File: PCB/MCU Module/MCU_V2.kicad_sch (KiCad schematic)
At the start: 11 parts, among them J2 Conn_01x09_Pin, J3 Conn_01x02_Socket, U1 XIAO-nRF54l15-SMD, U5 MAX17048G_T10

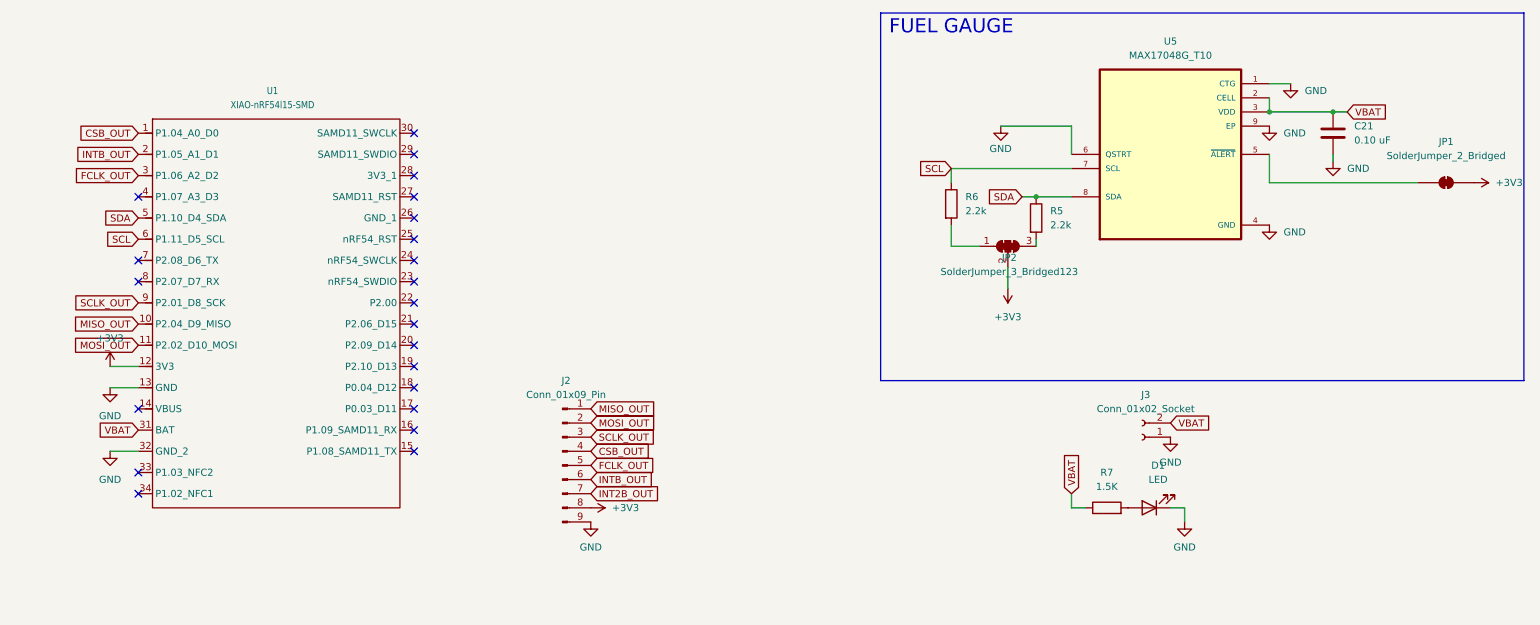
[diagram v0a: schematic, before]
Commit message: jogeshwari
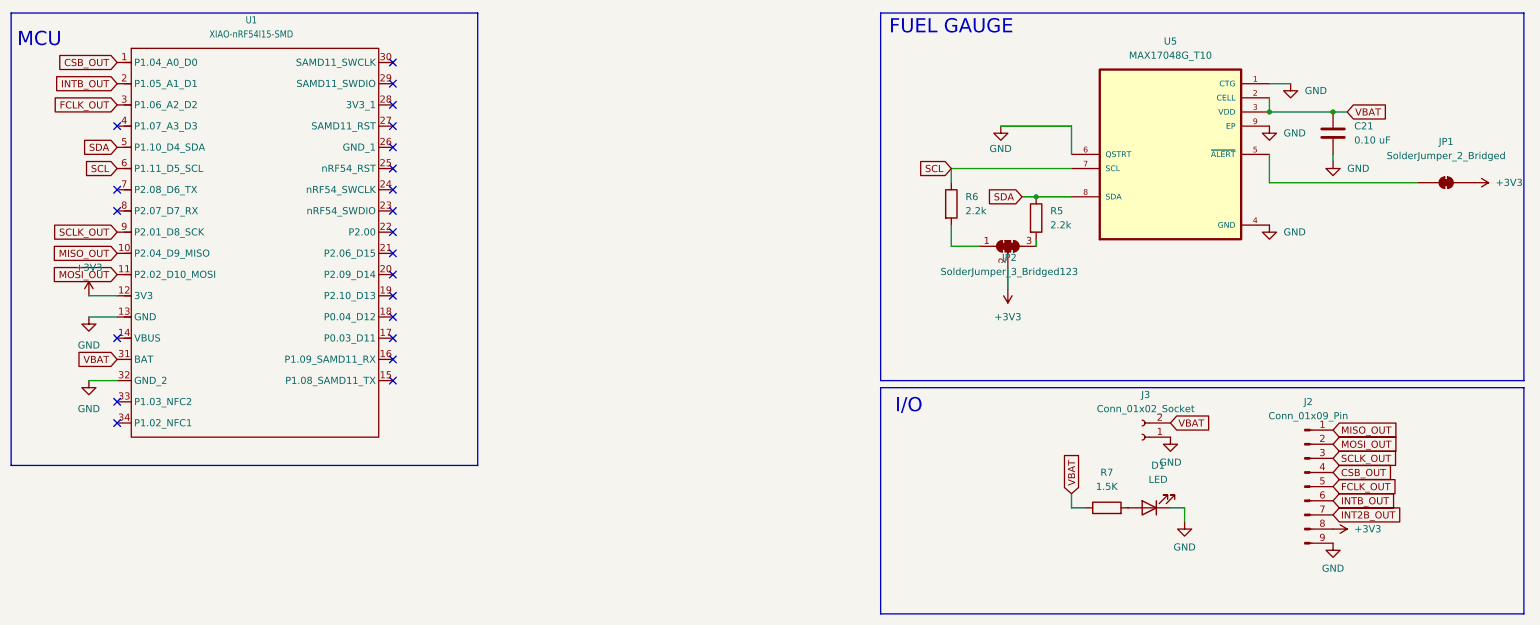
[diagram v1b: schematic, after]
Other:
- note added: "I/O"
- note added: "MCU"
- moved on the sheet: J2, U1
